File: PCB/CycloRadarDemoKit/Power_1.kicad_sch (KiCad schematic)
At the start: 33 parts, among them J401 20-16V Supply Voltage, Q401 SI2309CDS, U401 INA3221, U402 RT8259, U403 AP63205WU

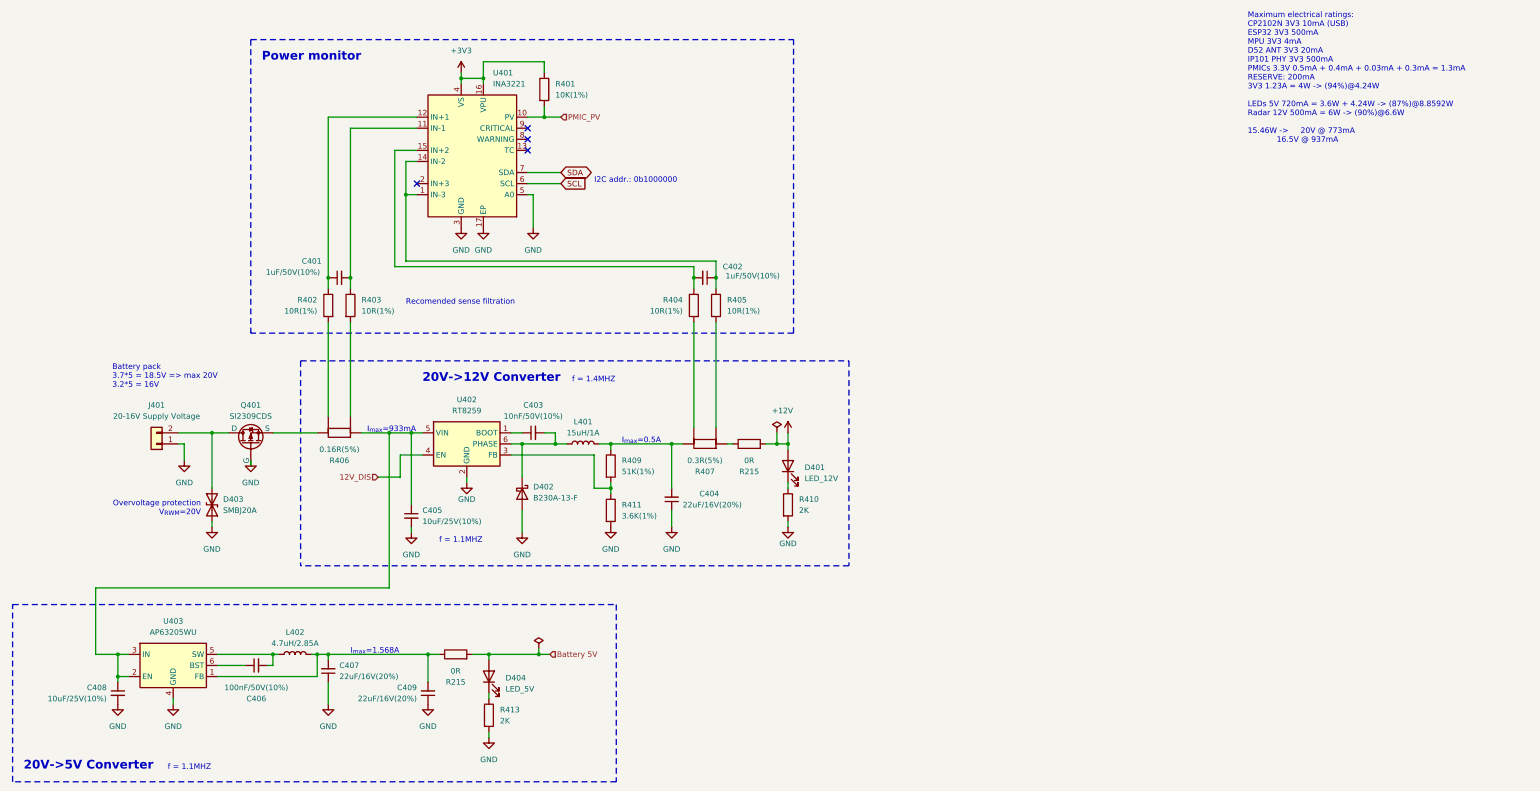
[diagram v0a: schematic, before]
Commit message: PCB small updates, schemtatic cosmetics, SEP FINAL
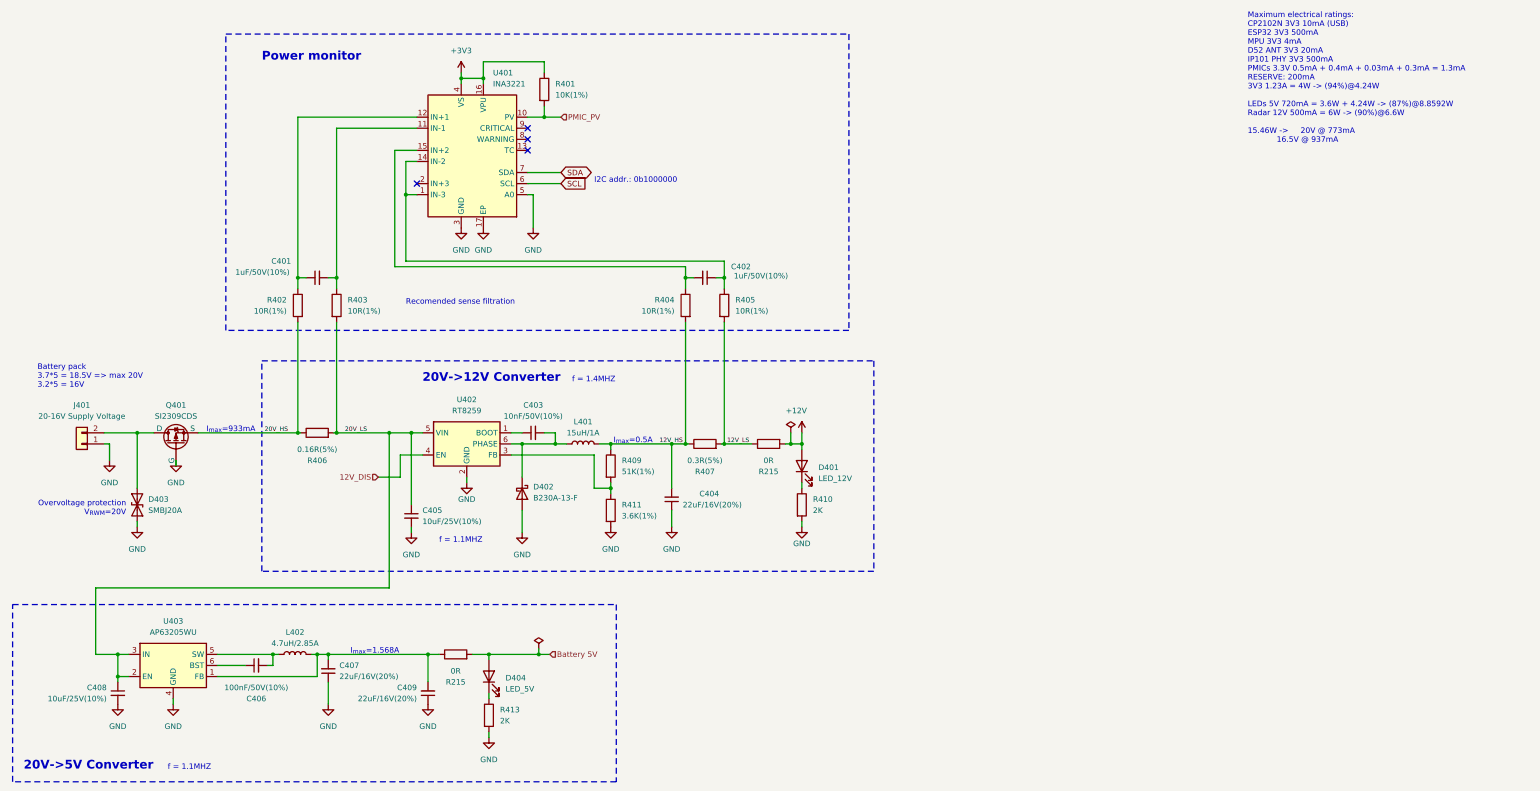
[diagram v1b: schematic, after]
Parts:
- R406, R407: symbol Analog:R_Shunt -> Device:R
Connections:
- net 20V_HS: now reaches Q401.3 (S), R406.1
- net 20V_HS: now also R402.2
- net 20V_LS: now reaches C405.1, C408.1, R406.2, U402.5 (VIN), U403.2 (EN), U403.3 (IN)
- net 20V_LS: now also R403.2
- net 12V_HS: now reaches C404.2, L401.2, R407.1, R409.1
- net 12V_HS: now also R404.2
- net 12V_LS: now reaches R215.1, R407.2
- net 12V_LS: now also R405.2
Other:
- moved on the sheet: C401, D401, D403, J401, Q401, R215, R402, R403, R404, R405, R410
